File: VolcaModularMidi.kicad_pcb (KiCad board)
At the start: 2 copper layers, 6 parts, among them J1 Conn_01x04_Male, J2 MIDI_IN, U1 6N139

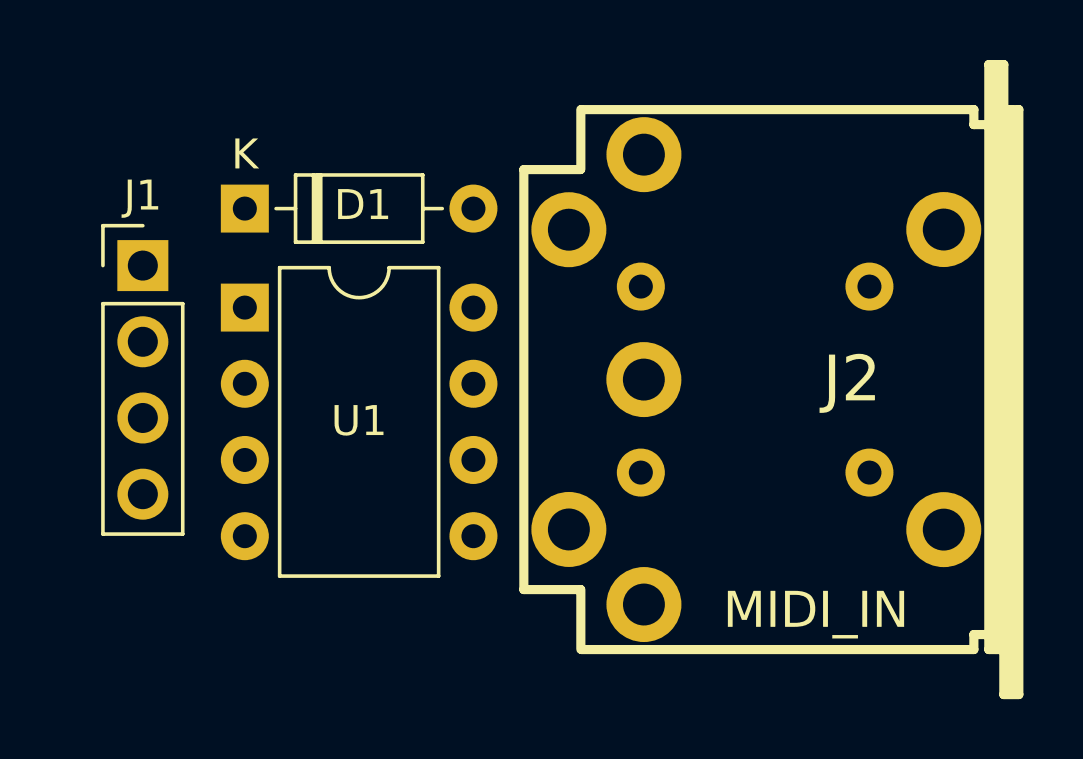
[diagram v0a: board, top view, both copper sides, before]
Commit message: Version 0.1 finished
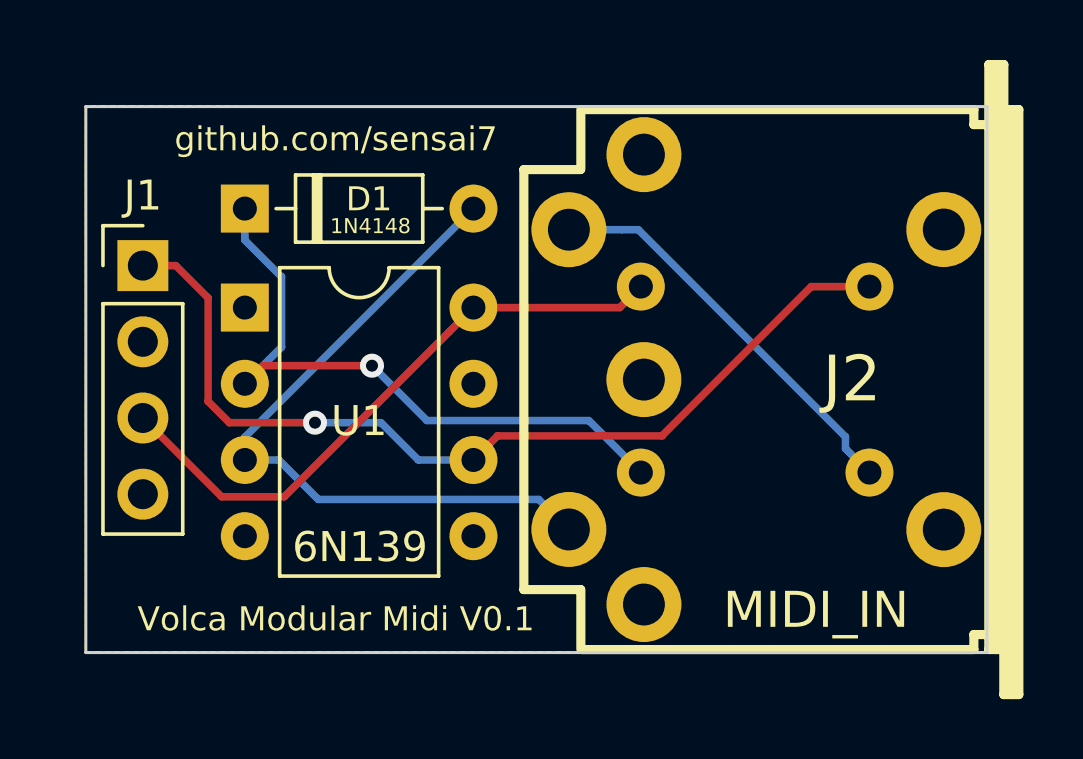
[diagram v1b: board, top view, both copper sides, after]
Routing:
- net RX: track 0.00 -> 31.3 mm, vias 0 -> 1
- net Net-(D1-Pad2): track 0.00 -> 23.3 mm
- net Net-(D1-Pad1): track 0.00 -> 21.8 mm, vias 0 -> 1
- net VCC: track 0.00 -> 20.6 mm
- net Net-(J2-Pad4): track 0.00 -> 13.6 mm
- added copper zone on B.Cu, net GND
- added copper zone on F.Cu, net GND
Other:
- board outline added: 30 x 18.2 mm
- net class Default: clearance 0.2 -> 0.3
- rule trace_clearance: 0.2 -> 0.3
- board text added: "+"
- board text added: "-"
- board text added: "R"
- board text added: "T"
- board text added: "Volca Modular Midi V0.1"
- board text added: "github.com/sensai7"
- board text removed: "VolcaModularMidi"
